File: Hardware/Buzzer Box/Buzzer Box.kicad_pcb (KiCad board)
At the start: 2 copper layers, 105.5 x 60.5 mm, 77 parts, among them IC1 4691, IC10 4691, IC11 4691, IC12 4691, IC2 4691, IC3 4691, IC4 4691, IC5 4691, IC6 4691, IC7 4691, IC8 4691, IC9 4691, J1 GPIO 2 + GND, J10 Conn_01x03_Socket, J11 USB_C_Receptacle_USB2.0_16P, J12 GPIO 2 + GND, J15 IO42, J16 IO41, J19 GND, J2 Conn_01x03_Socket, J20 3V3, J21 24V, J22 5V, J3 Conn_01x03_Socket, J4 Conn_01x03_Socket, J5 Conn_01x03_Socket, J6 GPIO 2 + GND, J7 Conn_01x03_Socket, J8 Conn_01x03_Socket, J9 Conn_01x03_Socket, Q1 AO3400A, Q2 AO3400A, Q3 AO3400A, Q4 AO3400A, Q5 AO3400A, Q6 AO3400A, Q7 AO3400A, Q8 AO3400A, U1 LTV-817S, U10 ESP32-S3-WROOM-1, U2 USBLC6-2SC6, U3 LTV-817S, U4 LTV-817S, U5 LTV-817S, U6 LTV-817S, U7 LTV-817S, U8 LTV-817S, U9 LTV-817S

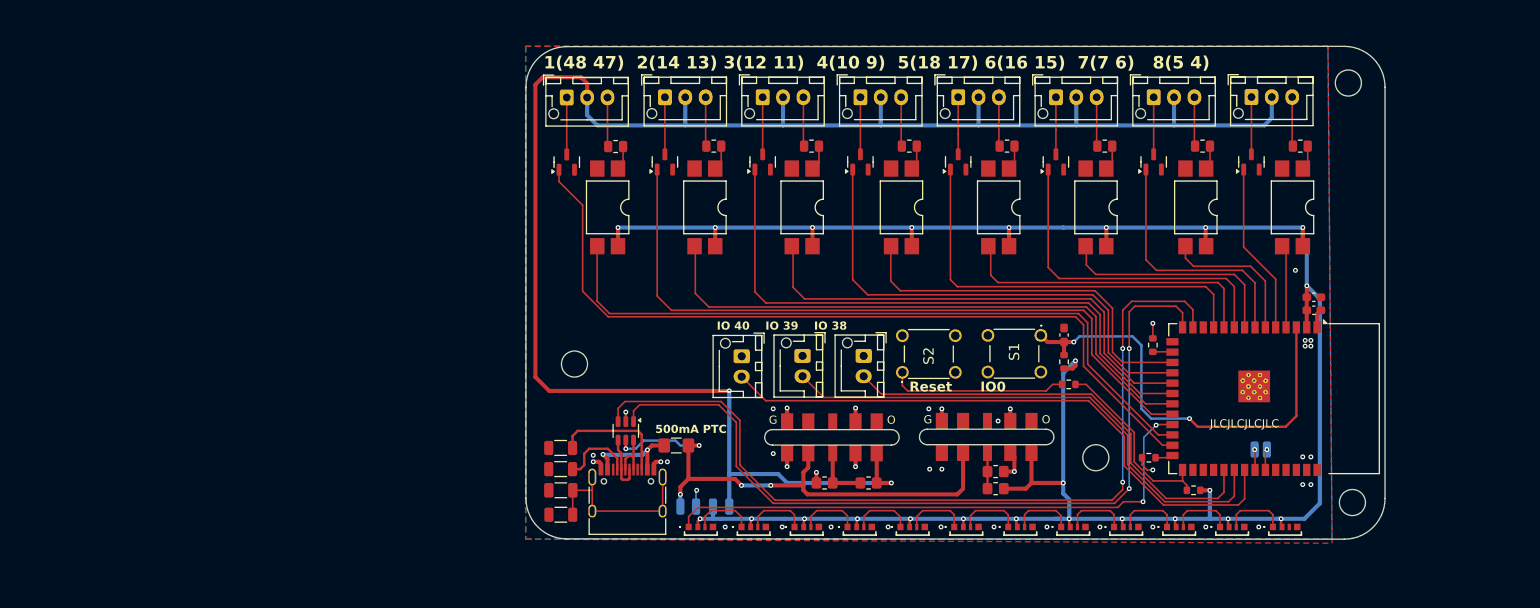
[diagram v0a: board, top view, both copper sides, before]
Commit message: Updated the PCB
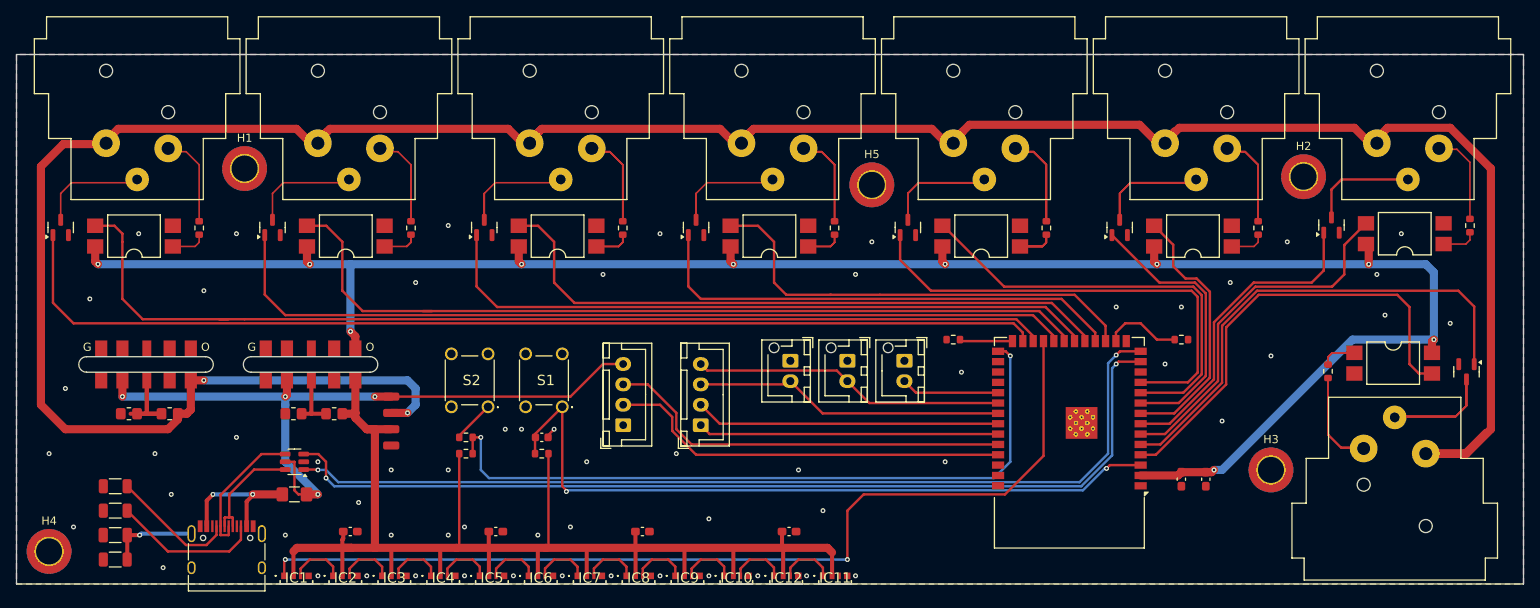
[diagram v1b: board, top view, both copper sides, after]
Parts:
- removed J10, J4, J5, J7, J8, J9: Conn_01x03_Socket, Connector_JST:JST_XH_B3B-XH-AM_1x03_P2.50mm_Vertical
- removed J15: IO42, Connector_Wire:SolderWirePad_1x01_SMD_1x2mm
- removed J16: IO41, Connector_Wire:SolderWirePad_1x01_SMD_1x2mm
- added C3: 100n, Capacitor_SMD:C_0603_1608Metric_Pad1.08x0.95mm_HandSolder, F.Cu at (119.8, 116.6)
- added C4: 100n, Capacitor_SMD:C_0603_1608Metric_Pad1.08x0.95mm_HandSolder, F.Cu at (137.8, 116.6)
- added C6: 100n, Capacitor_SMD:C_0603_1608Metric_Pad1.08x0.95mm_HandSolder, F.Cu at (101.8, 116.6)
- added C7: 100n, Capacitor_SMD:C_0603_1608Metric_Pad1.08x0.95mm_HandSolder, F.Cu at (84.0, 116.6)
- added H1: MountingHole_Pad, MountingHole:MountingHole_3.2mm_M3_ISO14580_Pad_TopBottom, F.Cu at (71.0, 72.0)
- added H2: MountingHole_Pad, MountingHole:MountingHole_3.2mm_M3_ISO14580_Pad_TopBottom, F.Cu at (201.0, 73.0)
- added H3: MountingHole_Pad, MountingHole:MountingHole_3.2mm_M3_ISO14580_Pad_TopBottom, F.Cu at (197.0, 109.0)
- added H4: MountingHole_Pad, MountingHole:MountingHole_3.2mm_M3_ISO14580_Pad_TopBottom, F.Cu at (47.0, 119.0)
- added H5: MountingHole_Pad, MountingHole:MountingHole_3.2mm_M3_ISO14580_Pad_TopBottom, F.Cu at (148.0, 74.0)
- added J13: NC3FAAH, Connector_Audio:Jack_XLR_Neutrik_NC3FAAH_Horizontal, F.Cu at (158.0, 68.9)
- added J14: NC3FAAH, Connector_Audio:Jack_XLR_Neutrik_NC3FAAH_Horizontal, F.Cu at (184.0, 68.9)
- added J17: NC3FAAH, Connector_Audio:Jack_XLR_Neutrik_NC3FAAH_Horizontal, F.Cu at (210.0, 68.9)
- added J18: NC3FAAH, Connector_Audio:Jack_XLR_Neutrik_NC3FAAH_Horizontal, F.Cu at (216.0, 107.0)
- added J23: NC3FAAH, Connector_Audio:Jack_XLR_Neutrik_NC3FAAH_Horizontal, F.Cu at (132.0, 68.9)
- added J24: NC3FAAH, Connector_Audio:Jack_XLR_Neutrik_NC3FAAH_Horizontal, F.Cu at (106.0, 68.9)
- added J25: NC3FAAH, Connector_Audio:Jack_XLR_Neutrik_NC3FAAH_Horizontal, F.Cu at (80.0, 68.9)
- added J26: NC3FAAH, Connector_Audio:Jack_XLR_Neutrik_NC3FAAH_Horizontal, F.Cu at (54.0, 68.9)
- C1: footprint Capacitor_SMD:C_0603_1608Metric_Pad1.08x0.95mm_HandSolder -> Capacitor_SMD:C_0603_1608Metric
- J19, J20, J22: moved to F.Cu
- J2: value Conn_01x03_Socket -> UART; footprint Connector_JST:JST_XH_B3B-XH-AM_1x03_P2.50mm_Vertical -> Connector_JST:JST_XH_B4B-XH-A_1x04_P2.50mm_Vertical
- J21: value 24V -> 24v; moved to F.Cu
- J3: value Conn_01x03_Socket -> JTAG; footprint Connector_JST:JST_XH_B3B-XH-AM_1x03_P2.50mm_Vertical -> Connector_JST:JST_XH_B4B-XH-A_1x04_P2.50mm_Vertical
- R10, R3, R4, R5, R6, R7, R8, R9: footprint Resistor_SMD:R_0805_2012Metric -> Resistor_SMD:R_0603_1608Metric
- moved R16 89.4 mm to (98.2, 107.0), turned to 0 degrees
- moved R20 86.5 mm to (77.0, 102.1), turned to 180 degrees
- moved R17 86.2 mm to (61.8, 102.1)
- moved R18 85.8 mm to (56.8, 102.1)
- moved U11 84.7 mm to (50.6, 97.0)
- moved U12 83.5 mm to (70.8, 97.0)
- moved R19 81.7 mm to (82.0, 102.1)
- moved R2 74.3 mm to (98.2, 105.0)
- moved J2 66.7 mm to (117.5, 103.5), turned to 90 degrees
- moved C1 65.3 mm to (107.5, 105.0), turned to 180 degrees
- moved R11 65.1 mm to (107.5, 107.0), turned to 0 degrees
- moved Q8 62.6 mm to (48.4, 79.2)
- moved S1 59.4 mm to (110.0, 101.2), turned to 180 degrees
- moved U9 58.3 mm to (57.4, 80.3), turned to 180 degrees
- moved IC11 55.6 mm to (143.5, 122.0)
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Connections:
- J2 pad 1: Net-(J2-Pin_1) -> GND
- J2 pad 2: +24V -> Net-(J2-Pin_2)
- J3 pad 2: +24V -> Net-(J3-Pin_2)
- J3 pad 3: Net-(J3-Pin_3) -> Net-(J12-Pin_2)
- Q1 pad 3: Net-(J3-Pin_1) -> Net-(Q1-D)
- Q2 pad 3: Net-(J2-Pin_1) -> Net-(Q2-D)
- R3 pad 1: Net-(J3-Pin_3) -> Net-(J13-Pad2)
- R4 pad 1: Net-(J2-Pin_3) -> Net-(J14-Pad2)
- U10 pad 34: Net-(J16-Pin_1) -> Net-(J3-Pin_2)
- U10 pad 35: Net-(J15-Pin_1) -> Net-(J3-Pin_1)
- U10 pad 36: unconnected-(U10-RXD0-Pad36) -> Net-(J2-Pin_3)
- U10 pad 37: unconnected-(U10-TXD0-Pad37) -> Net-(J2-Pin_2)
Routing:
- net +3.3V: track 274.1 -> 406.5 mm, vias 24 -> 10
- net +24V: track 220.3 -> 342.2 mm
- net Net-(U10-IO0): track 22.9 -> 88.0 mm, vias 0 -> 2
- net Net-(J2-Pin_2): track 0.00 -> 49.6 mm
- net Net-(IC1-DIN): track 69.9 -> 118.0 mm
- net /taster IO3/Taster: track 10.2 -> 56.1 mm
- net Net-(J2-Pin_3): track 6.04 -> 50.2 mm
- net Net-(J6-Pin_2): track 55.6 -> 12.1 mm
- net /taster IO7/Taster: track 87.1 -> 127.2 mm
- net /taster IO3/LED: track 21.0 -> 60.7 mm
- net Net-(J3-Pin_2): track 0.00 -> 37.5 mm
- net Net-(Q2-D): track 0.00 -> 37.1 mm
- net Net-(J14-Pad2): track 0.00 -> 36.7 mm
- net Net-(J13-Pad2): track 0.00 -> 36.7 mm
- net Net-(S1-COM_1): track 54.2 -> 90.2 mm
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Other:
- board size 105.5 x 60.5 mm -> 185 x 65 mm
- board text removed: "1(48 47) 2(14 13) 3(12 11) 4(10 9) 5(18 17) 6(16 15) 7(7 6) 8(5 4)"
- board text removed: "IO 40 IO 39 IO 38"
- board text removed: "JLCJLCJLCJLC"
- board text removed: "Reset IO0"
